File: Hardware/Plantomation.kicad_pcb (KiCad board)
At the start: 2 copper layers, 100 x 80 mm, 97 parts, among them J1 12V, J10 ADC1_0, J11 Valve 3, J12 Valve 4, J13 Ch_Sel, J14 GSD090012SEU, J2 USB_B, J3 ADC1_4, J4 ADC1_5, J5 ADC1_6, J6 ADC1_7, J7 PeriPump, J8 Valve 1, J9 Valve 2, Q1 BC846, Q2 DMG1012UW7, Q3 BC846, Q4 BSS138, Q5 BSS138, Q6 BSS138, Q7 BSS138, SW1 RST, SW2 BOOT, U1 ESP32-WROOM-32, U2 USBLC6-2SC6, U3 L7805, U4 AMS1117-3.3, U5 CP2102N-Axx-xQFN28

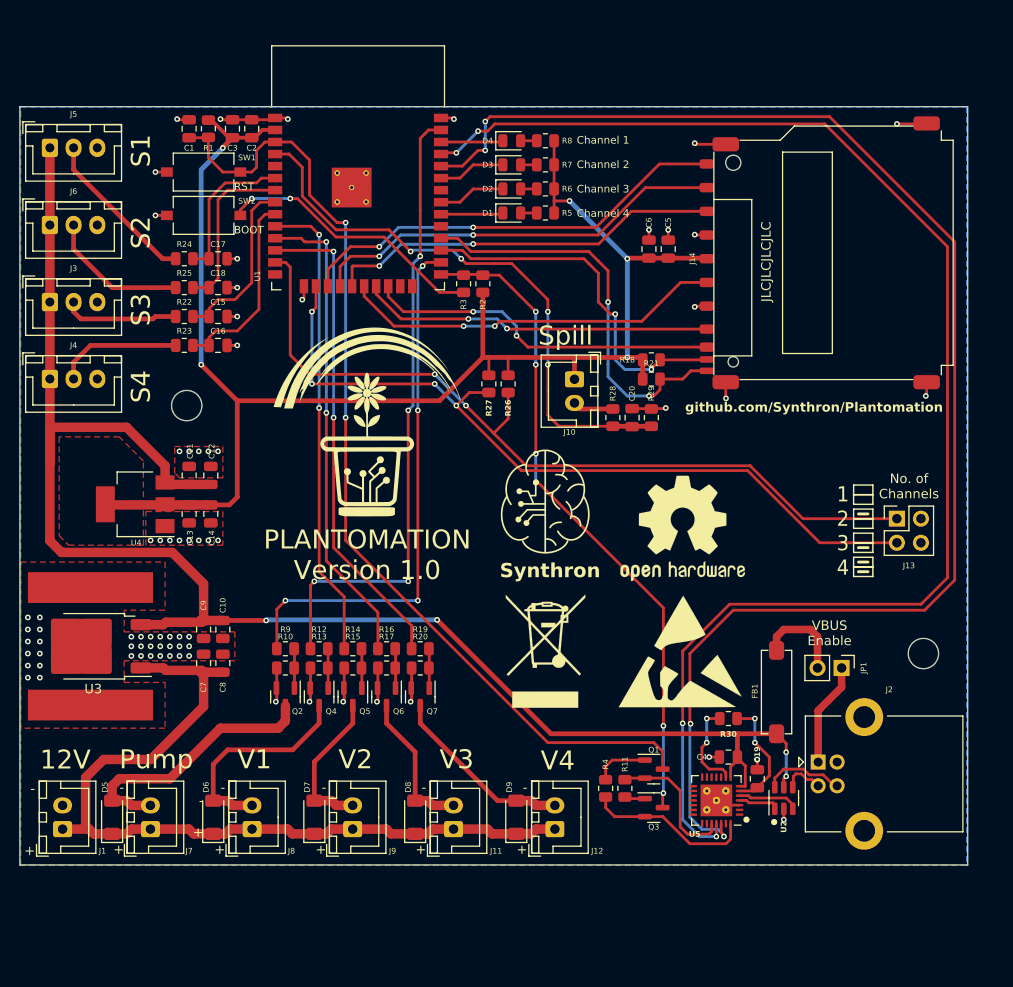
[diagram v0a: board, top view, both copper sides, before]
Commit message: Big Repo Overhaul Started Documentation First Review Overhaul of Schematic and Layout First working Test Code for webpage and OTA
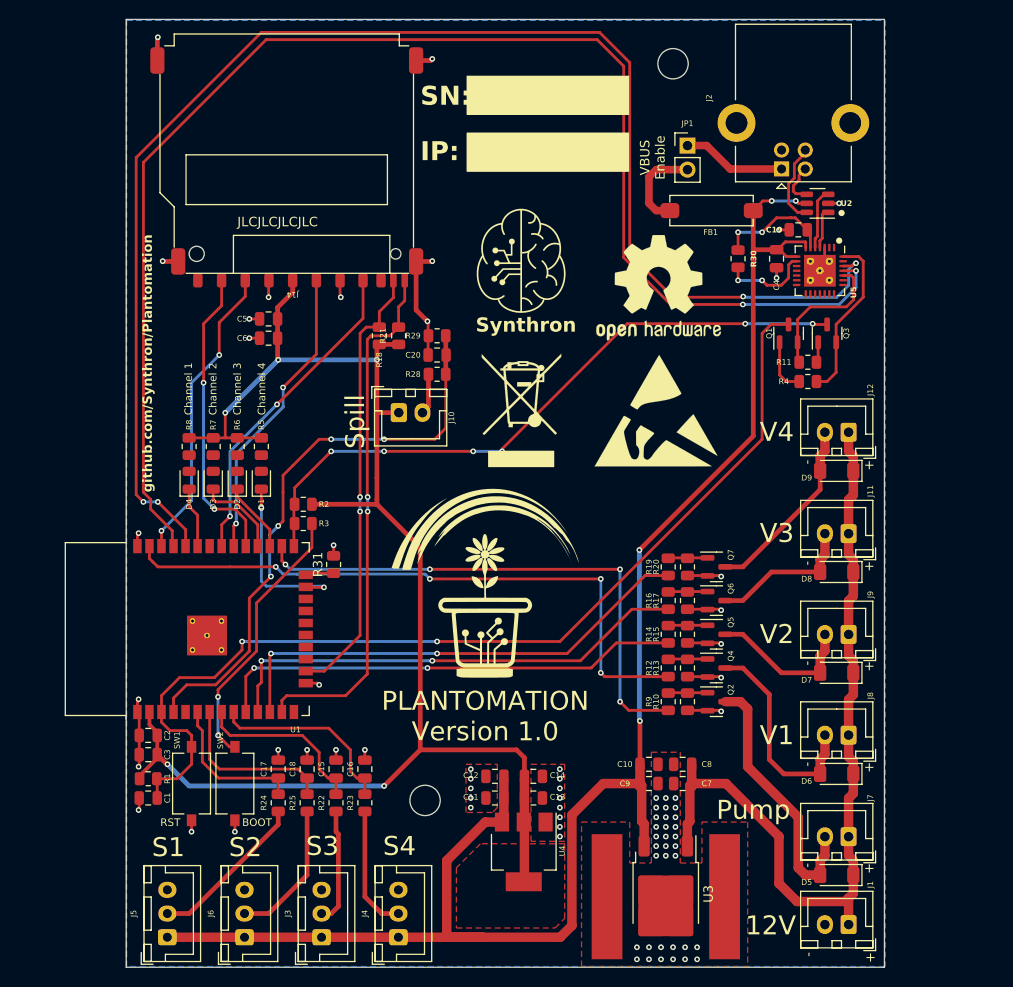
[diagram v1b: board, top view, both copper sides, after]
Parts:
- removed J13: Ch_Sel, Connector_PinHeader_2.54mm:PinHeader_2x02_P2.54mm_Vertical
- removed R26, R27: 1k, Resistor_SMD:R_0805_2012Metric
- added R31: 4k7, Resistor_SMD:R_0805_2012Metric, F.Cu at (133.1, 98.3)
- R11, R4: value 100 -> 4k7
- moved J5 84.2 mm to (115.6, 137.6), turned to 90 degrees
- moved J1 83.5 mm to (187.4, 136.3), turned to 180 degrees
- moved J6 77.9 mm to (123.7, 137.6), turned to 90 degrees
- moved D5 76.7 mm to (186.2, 131.1), turned to 180 degrees
- moved J7 73.7 mm to (187.4, 127.0), turned to 180 degrees
- moved J3 72.9 mm to (131.8, 137.6), turned to 90 degrees
- moved C1 70.7 mm to (113.5, 122.9), turned to 180 degrees
- moved J4 69.4 mm to (139.9, 137.6), turned to 90 degrees
- moved R1 68.9 mm to (113.5, 120.9), turned to 0 degrees
- moved H2 67.6 mm to (168.9, 45.5), turned to 90 degrees
- moved C3 66.6 mm to (113.5, 118.4), turned to 180 degrees
- moved HS1 66.2 mm to (168.1, 133.3), turned to 180 degrees
- moved D6 65.9 mm to (186.2, 120.4), turned to 180 degrees
- moved U3 65.8 mm to (168.1, 133.1), turned to -90 degrees
- moved C2 64.9 mm to (113.5, 116.3), turned to 180 degrees
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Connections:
- net Net-(U1-IO32) renamed /Sensor3
- net Net-(U1-IO33) renamed /Sensor4
- net Net-(U1-IO34) renamed /Sensor1
- net Net-(U1-IO35) renamed /Sensor2
- net PeriPump renamed Pump
- J14 pad 1: SD3 -> VSPI_CS
- J14 pad 2: CMD -> VSPI_MOSI
- J14 pad 5: CLK -> VSPI_CLK
- J14 pad 7: SD0 -> VSPI_MISO
- J14 pad 8: SD1 -> unconnected-(J14-DAT1-Pad8)
- J14 pad 9: SD2 -> unconnected-(J14-DAT2-Pad9)
- U1 pad 13: Net-(J13-Pin_1) -> ~{Protect}
- U1 pad 16: Net-(J13-Pin_3) -> ~{Detect}
- U1 pad 17: SD2 -> unconnected-(U1-SHD/SD2-Pad17)
- U1 pad 18: SD3 -> unconnected-(U1-SWP/SD3-Pad18)
- U1 pad 19: CMD -> unconnected-(U1-SCS/CMD-Pad19)
- U1 pad 20: CLK -> unconnected-(U1-SCK/CLK-Pad20)
- U1 pad 21: SD0 -> unconnected-(U1-SDO/SD0-Pad21)
- U1 pad 22: SD1 -> unconnected-(U1-SDI/SD1-Pad22)
- U1 pad 23: unconnected-(U1-IO15-Pad23) -> Ch4_Led
- U1 pad 24: unconnected-(U1-IO2-Pad24) -> Net-(U1-IO2)
- U1 pad 27: ~{Detect} -> Ch3_Led
- U1 pad 28: ~{Protect} -> Ch2_Led
- U1 pad 29: unconnected-(U1-IO5-Pad29) -> VSPI_CS
- U1 pad 30: Ch4_Led -> VSPI_CLK
- U1 pad 31: Ch3_Led -> VSPI_MISO
- U1 pad 33: Ch2_Led -> Ch1_Led
- U1 pad 36: Ch1_Led -> VSPI_MOSI
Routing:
- net Net-(J13-Pin_1): track 87.2 -> 0.00 mm, vias 2 -> 0
- net Net-(J13-Pin_3): track 83.1 -> 0.00 mm, vias 4 -> 0
- net SD2: track 46.4 -> 0.00 mm, vias 2 -> 0
- net SD3: track 44.2 -> 0.00 mm, vias 2 -> 0
- net CMD: track 41.9 -> 0.00 mm, vias 2 -> 0
- net CLK: track 40.4 -> 0.00 mm, vias 2 -> 0
- net SD1: track 37.5 -> 0.00 mm, vias 2 -> 0
- net SD0: track 37.2 -> 0.00 mm, vias 2 -> 0
- net VSPI_MISO: track 0.00 -> 34.2 mm, vias 0 -> 2
- net VSPI_CS: track 0.00 -> 31.9 mm, vias 0 -> 2
- net VSPI_MOSI: track 0.00 -> 31.7 mm, vias 0 -> 2
- net VSPI_CLK: track 0.00 -> 31.7 mm, vias 0 -> 2
- net ~{Protect}: track 43.2 -> 55.8 mm
- net Ch4_Led: track 6.58 -> 18.5 mm, vias 0 -> 2
- net ~{Detect}: track 38.4 -> 47.0 mm
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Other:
- board size 100 x 80 mm -> 80 x 100 mm
- board text added: "IP:"
- board text added: "SN:"
- board text removed: "1 2 3 4"
- board text removed: "No. of Channels"
